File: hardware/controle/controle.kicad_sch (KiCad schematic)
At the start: 38 parts, among them J3 PWR, J4 DATA, J5 UART7, J6 TWI3, J7 SENS0375, J8 TWI4, J9 LED, U2 MCP7940N-xSN, U4 ULN2003, Y1 32.768Khz

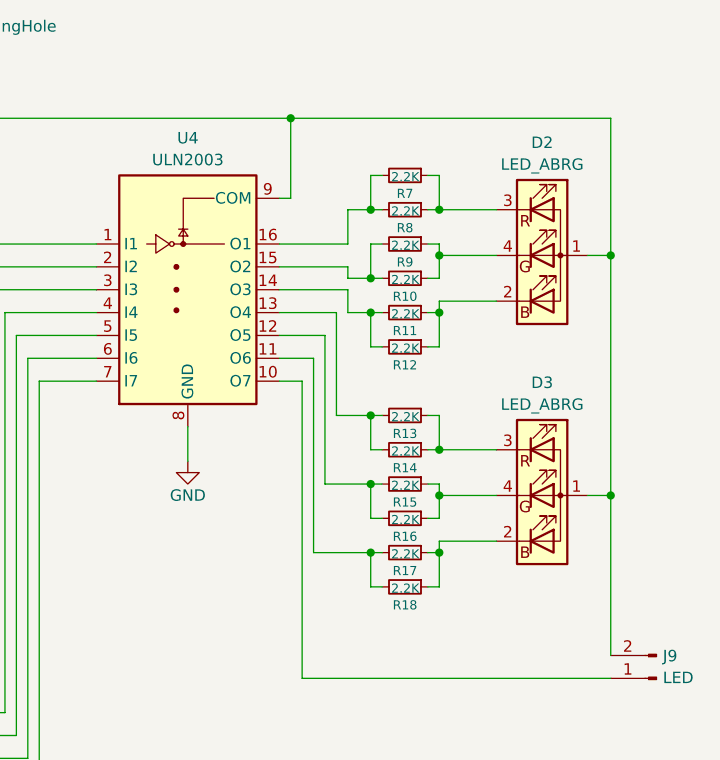
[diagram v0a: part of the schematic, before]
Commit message: Update LED resistors values. Minor updates to PCB
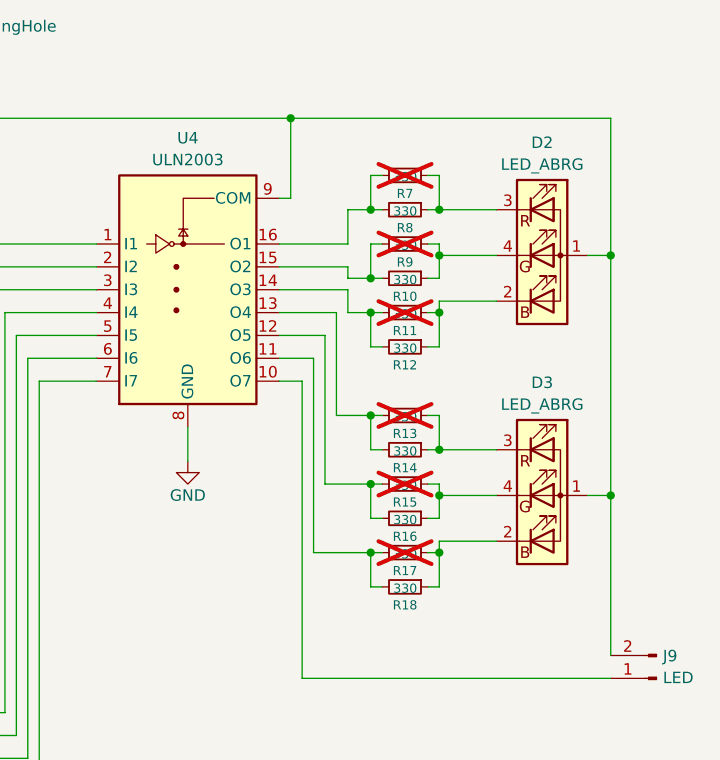
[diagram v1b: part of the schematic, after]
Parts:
- R10, R12, R14, R16, R18, R8: value 2.2K -> 330
- R11, R13, R15, R17, R7, R9: value 2.2K -> 330; now not fitted
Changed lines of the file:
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@@
 		(in_bom yes)
 		(on_board yes)
-		(dnp no)
+		(dnp yes)
 		(property "Reference" "R11"
 			(at 217.17 61.722 90)
@@
 			)
 		)
-		(property "Value" "2.2K"
+		(property "Value" "330"
 			(at 217.1954 59.8678 90)
 			(effects
@@
 			)
 		)
-		(property "Value" "2.2K"
+		(property "Value" "330"
 			(at 217.1954 75.1078 90)
 			(effects
@@
 		(in_bom yes)
 		(on_board yes)
-		(dnp no)
+		(dnp yes)
 		(property "Reference" "R7"
 			(at 217.17 46.482 90)
@@
 			)
 		)
-		(property "Value" "2.2K"
+		(property "Value" "330"
 			(at 217.1954 44.6278 90)
 			(effects
@@
 			)
 		)
-		(property "Value" "2.2K"
+		(property "Value" "330"
 			(at 217.1954 82.7278 90)
 			(effects
@@
 		(in_bom yes)
 		(on_board yes)
-		(dnp no)
+		(dnp yes)
 		(property "Reference" "R9"
 			(at 217.17 54.102 90)
@@
 			)
 		)
-		(property "Value" "2.2K"
+		(property "Value" "330"
 			(at 217.1954 52.2478 90)
 			(effects
@@
 			)
 		)
-		(property "Value" "2.2K"
+		(property "Value" "330"
 			(at 217.1954 56.0578 90)
 			(effects
@@
 			)
 		)
-		(property "Value" "2.2K"
+		(property "Value" "330"
 			(at 217.1954 90.3478 90)
 			(effects
@@
 		(in_bom yes)
 		(on_board yes)
-		(dnp no)
+		(dnp yes)
 		(property "Reference" "R13"
 			(at 217.17 73.152 90)
@@
 			)
 		)
-		(property "Value" "2.2K"
+		(property "Value" "330"
 			(at 217.1954 71.2978 90)
 			(effects
@@
 		(in_bom yes)
 		(on_board yes)
-		(dnp no)
+		(dnp yes)
 		(property "Reference" "R15"
 			(at 217.17 80.772 90)
@@
 			)
 		)
-		(property "Value" "2.2K"
+		(property "Value" "330"
 			(at 217.1954 78.9178 90)
 			(effects
@@
 			)
 		)
-		(property "Value" "2.2K"
+		(property "Value" "330"
 			(at 217.1954 63.6778 90)
 			(effects
@@
 			)
 		)
-		(property "Value" "2.2K"
+		(property "Value" "330"
 			(at 217.1954 48.4378 90)
 			(effects
@@
 		(in_bom yes)
 		(on_board yes)
-		(dnp no)
+		(dnp yes)
 		(property "Reference" "R17"
 			(at 217.17 88.392 90)
@@
 			)
 		)
-		(property "Value" "2.2K"
+		(property "Value" "330"
 			(at 217.1954 86.5378 90)
 			(effects
